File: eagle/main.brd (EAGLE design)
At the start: 49.5 x 49.5 mm, 43 parts, among them Q1 SQJ886EP, U1 LTC3789EGNPBF

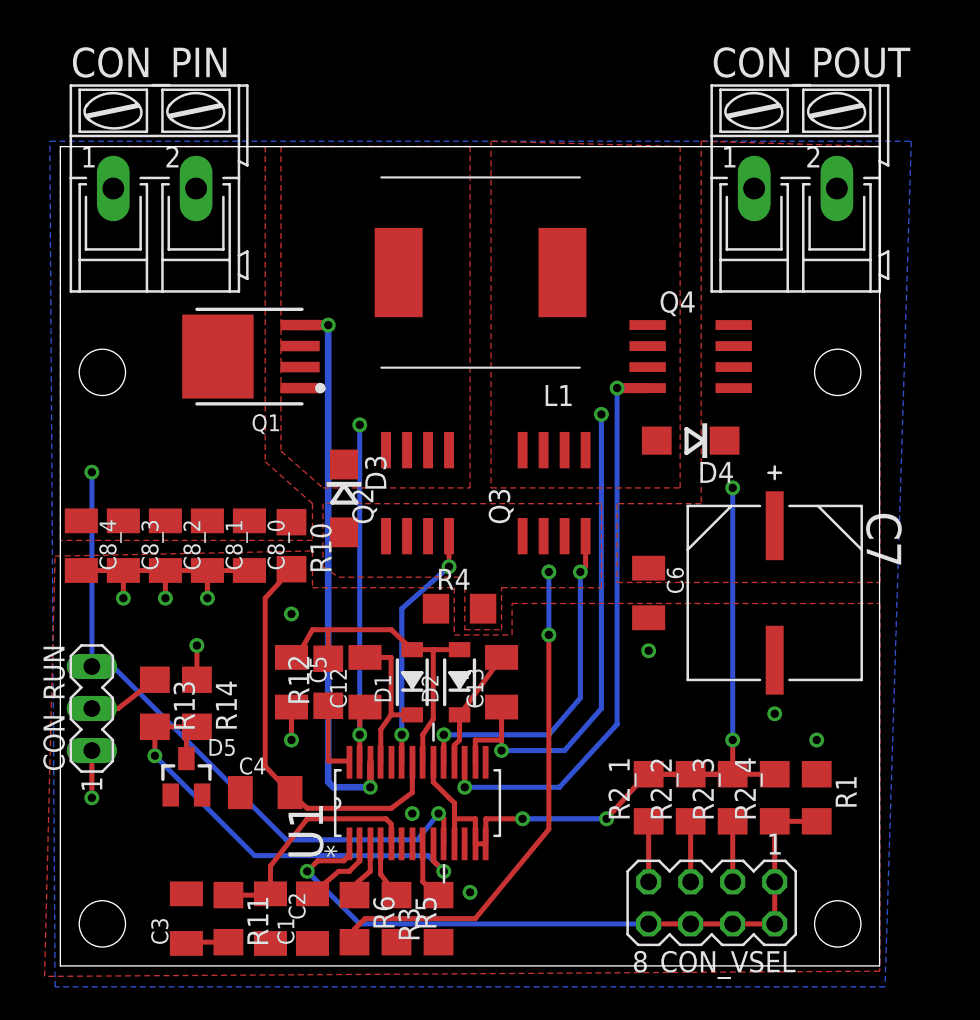
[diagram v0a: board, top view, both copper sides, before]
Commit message: [ update ] sch
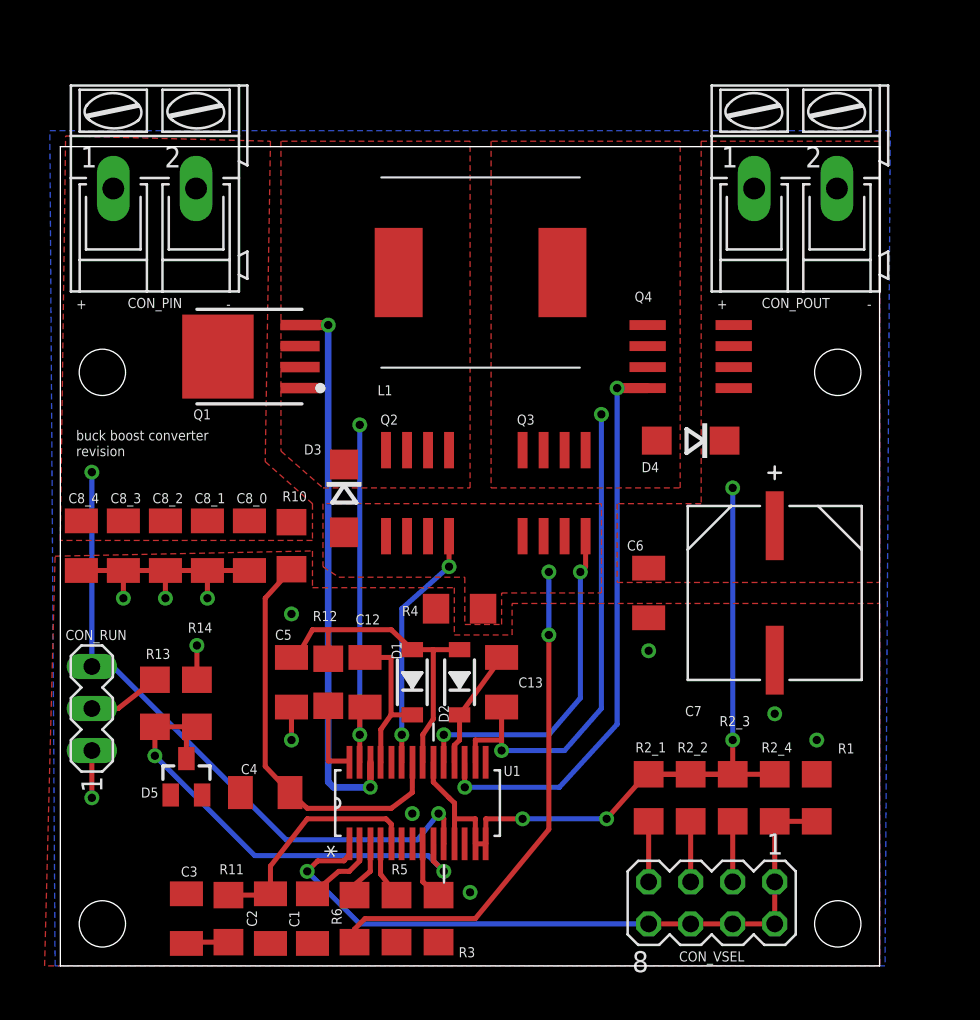
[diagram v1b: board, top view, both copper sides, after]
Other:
- board text added: "+"
- board text added: "-"
- board text added: "buck boost converter"
- board text added: "revision"
